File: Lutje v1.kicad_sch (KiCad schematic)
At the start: 24 parts, among them J1 Conn_01x02, J2 Conn_Coaxial, J3 Conn_01x02, J4 Conn_01x02, J5 Conn_01x02, U1 SX1280, U11 DRV8212DRL, U12 DRV8212DRL, U2 2450FM07D0034, U3 ESP32-S3S3FN8, U7 DRV8212DRL, U8 AMS1117-3.3, Y1 XC21M4-52.000-F10NNHPL

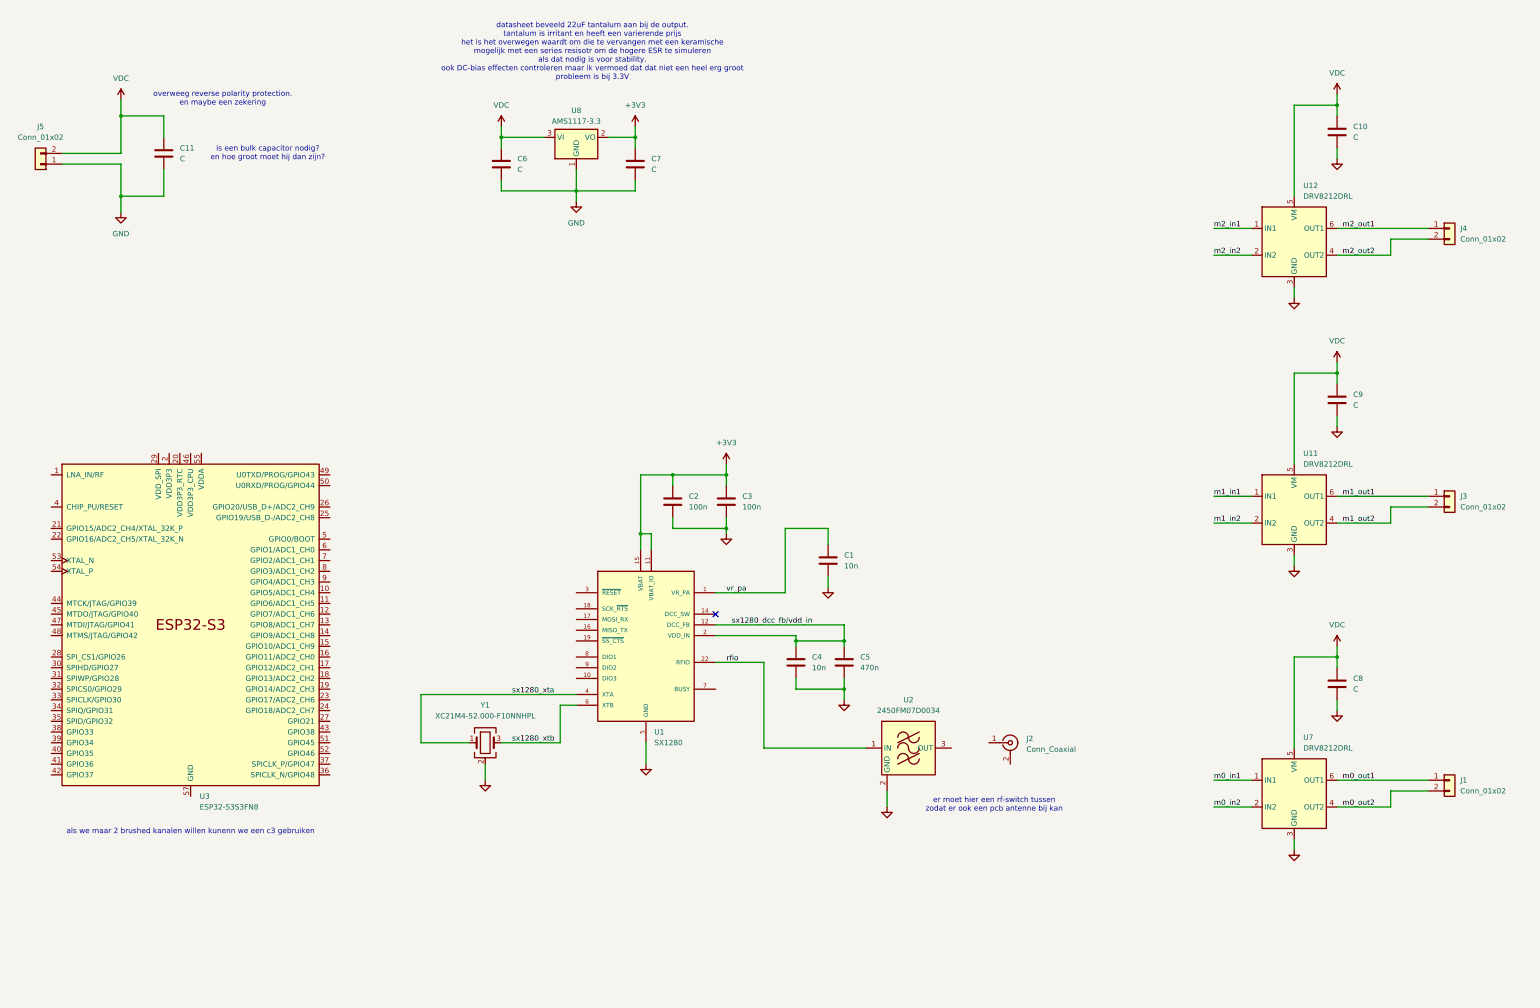
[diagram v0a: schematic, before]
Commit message: begin esp inrichting gemaakt
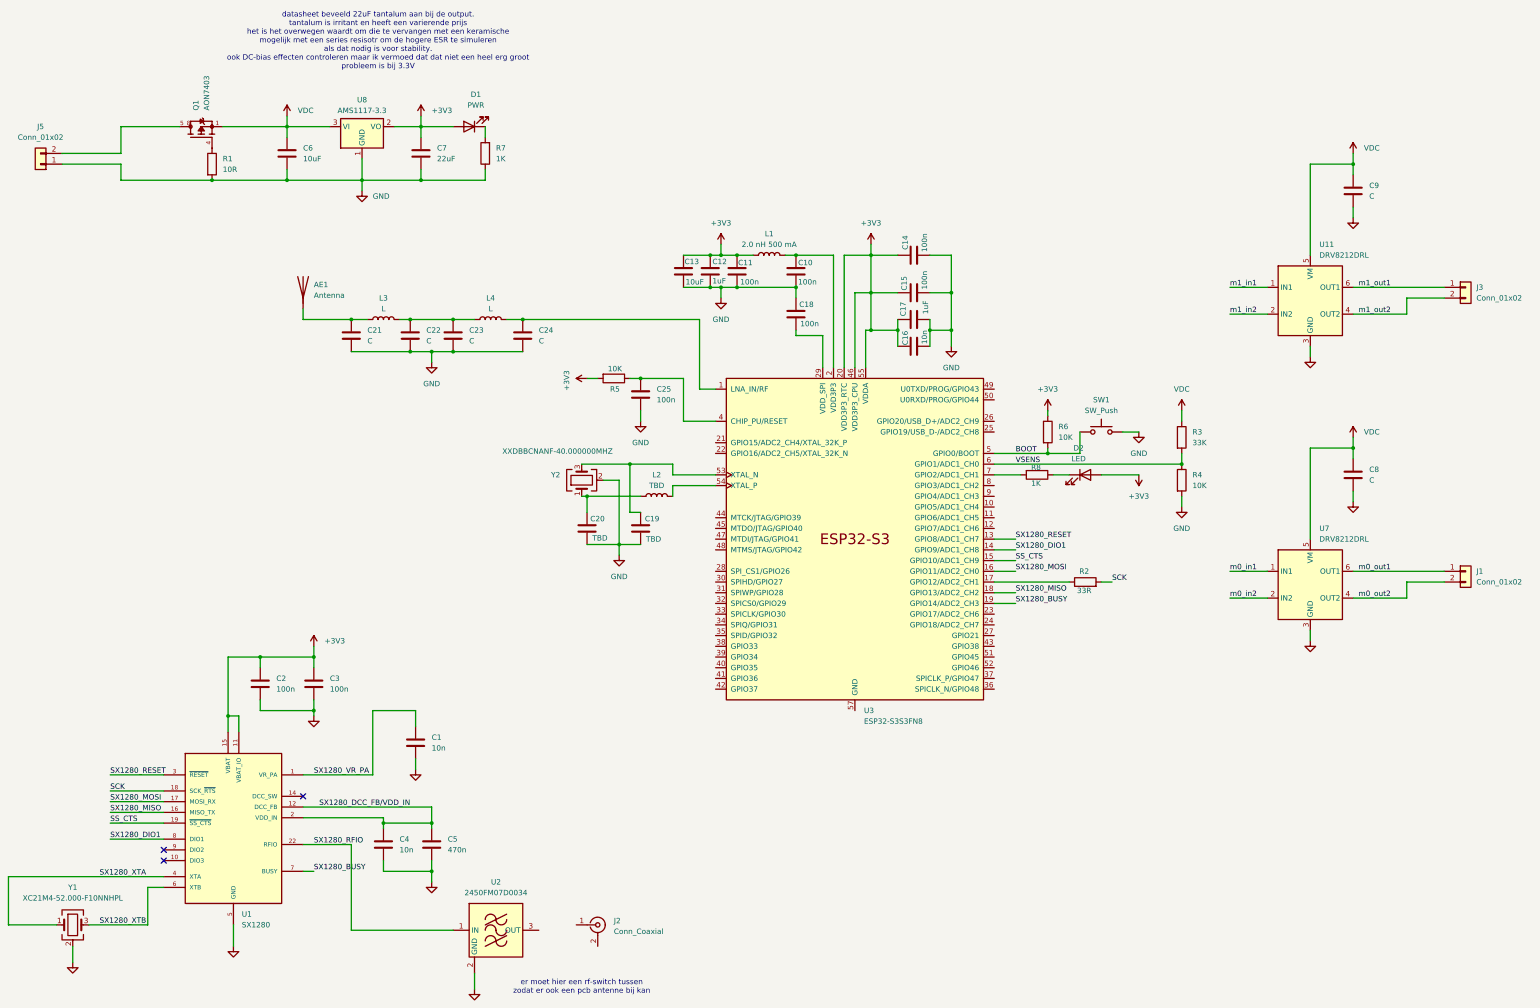
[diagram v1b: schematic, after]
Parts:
- removed J4: Conn_01x02, symbol Connector_Generic:Conn_01x02
- removed U12: DRV8212DRL, Package_TO_SOT_SMD:SOT-563, symbol .local:DRV8212DRL
- added AE1: Antenna, symbol Device:Antenna
- added C12, C17: 1uF, symbol Device:C
- added C13: 10uF, symbol Device:C
- added C14, C15, C18, C25: 100n, symbol Device:C
- added C16: 10n, symbol Device:C
- added C19, C20: TBD, symbol Device:C
- added C21, C22, C23, C24: C, symbol Device:C
- added D1: PWR, symbol Device:LED
- added D2: LED, symbol Device:LED
- added L1: 2.0 nH 500 mA, symbol Device:L
- added L2: TBD, symbol Device:L
- added L3, L4: L, symbol Device:L
- added Q1: AON7403, AON7403:TRANS_AON7403, symbol AON7403:AON7403
- added R1: 10R, symbol Device:R
- added R2: 33R, symbol Device:R
- added R3: 33K, symbol Device:R
- added R4, R5, R6: 10K, symbol Device:R
- added R7, R8: 1K, symbol Device:R
- added SW1: SW_Push, symbol Switch:SW_Push
- added Y2: XXDBBCNANF-40.000000MHZ, symbol Device:Crystal_GND24
- C10, C11: value C -> 100n
- C6: value C -> 10uF
- C7: value C -> 22uF
- J2: footprint Connector_Coaxial:U.FL_Hirose_U.FL-R-SMT-1_Vertical -> (none)
- Y1: lcsc C3034316 -> (none)
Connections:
- net +3V3: now also C11.1, U3.20 (VDD3P3_RTC), U3.46 (VDD3P3_CPU), U3.55 (VDDA), U3.56 (VDDA), C12.1, C13.1, C14.2, C15.2, C16.2, C17.2, D1.2 (A), D2.2 (A), L1.1, R5.2, R6.1
- net GND: now also C12.2, C13.2, C14.1, C15.1, C16.1, C17.1, C18.1, C19.2, C20.2, C21.2, C22.2, C23.2, C24.2, C25.2, R1.2, R4.2, R7.1, SW1.2, Y2.2 (G), Y2.4 (G)
- net VDC: now also Q1.1, Q1.2, Q1.3, R3.1; no longer C10.1, C11.1, J5.2 (Pin_2)
- net VDD3P3: now also C10.1, L1.2
- net at U3.1 (LNA_IN/RF): now also C24.1, L4.2
- net SX1280_RESET: now reaches U3.13 (GPIO8/ADC1_CH7)
- net SX1280_RESET: now also U1.3 (~{RESET})
- net SX1280_DIO1: now reaches U3.14 (GPIO9/ADC1_CH8)
- net SX1280_DIO1: now also U1.8 (DIO1)
- net SS_CTS: now reaches U3.15 (GPIO10/ADC1_CH9)
- net SS_CTS: now also U1.19 (~{SS_CTS})
- net SX1280_MOSI: now reaches U3.16 (GPIO11/ADC2_CH0)
- net SX1280_MOSI: now also U1.17 (MOSI_RX)
- net at U3.17 (GPIO12/ADC2_CH1): now also R2.1
- net SX1280_MISO: now reaches U3.18 (GPIO13/ADC2_CH2)
- net SX1280_MISO: now also U1.16 (MISO_TX)
- net SX1280_BUSY: now reaches U3.19 (GPIO14/ADC2_CH3)
- net SX1280_BUSY: now also U1.7 (BUSY)
- net at U3.29 (VDD_SPI): now also C18.2
- net at U3.4 (CHIP_PU/RESET): now also C25.1, R5.1
- net BOOT: now reaches U3.5 (GPIO0/BOOT)
- net BOOT: now also R6.2, SW1.1
- net at U3.53 (XTAL_N): now also C19.1, Y2.3
- net at U3.54 (XTAL_P): now also L2.2
- net VSENS: now reaches U3.6 (GPIO1/ADC1_CH0)
- net VSENS: now also R3.2, R4.1
- net at U3.7 (GPIO2/ADC1_CH1): now also R8.2
- net SCK: now reaches U1.18 (SCK_~{RTS})
- net SCK: now also R2.2
- net rfio renamed SX1280_RFIO
- net sx1280_dcc_fb/vdd_in renamed SX1280_DCC_FB/VDD_IN
- net sx1280_xta renamed SX1280_XTA
- net sx1280_xtb renamed SX1280_XTB
- net vr_pa renamed SX1280_VR_PA
- new net: C22.1, C23.1, L3.2, L4.1
- new net: C20.1, L2.1, Y2.1
- new net: AE1.1 (A), C21.1, L3.1
- new net: D1.1 (K), R7.2
- new net: Q1.4, R1.1
- new net: J5.2 (Pin_2), Q1.5_8
- new net: D2.1 (K), R8.1
- no-connect marks 1 -> 3
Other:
- note removed: "als we maar 2 brushed kanalen willen kunenn we een c3 gebruiken"
- note removed: "is een bulk capacitor nodig? en hoe groot moet hij dan zijn?"
- note removed: "overweeg reverse polarity protection. en maybe een zekering"
- moved on the sheet: C1, C2, C3, C4, C5, C8, C9, J1, J2, J3, U1, U11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
